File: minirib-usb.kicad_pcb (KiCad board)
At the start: 2 copper layers, 79.5 x 23 mm, 59 parts, among them J1 USB_B_Micro, J2 Mini-DIN-6-Shielded, J3 RS232, Q1 MMBT3906, Q2 MMBT3904, Q3 MMBT3904, Q4 MMBT3904, Q5 MMBT3906, Q6 MMBT3904, Q7 MMBT3904, Q8 BSS138W, U1 FT231XS, U2 TL071, U3 MAX232

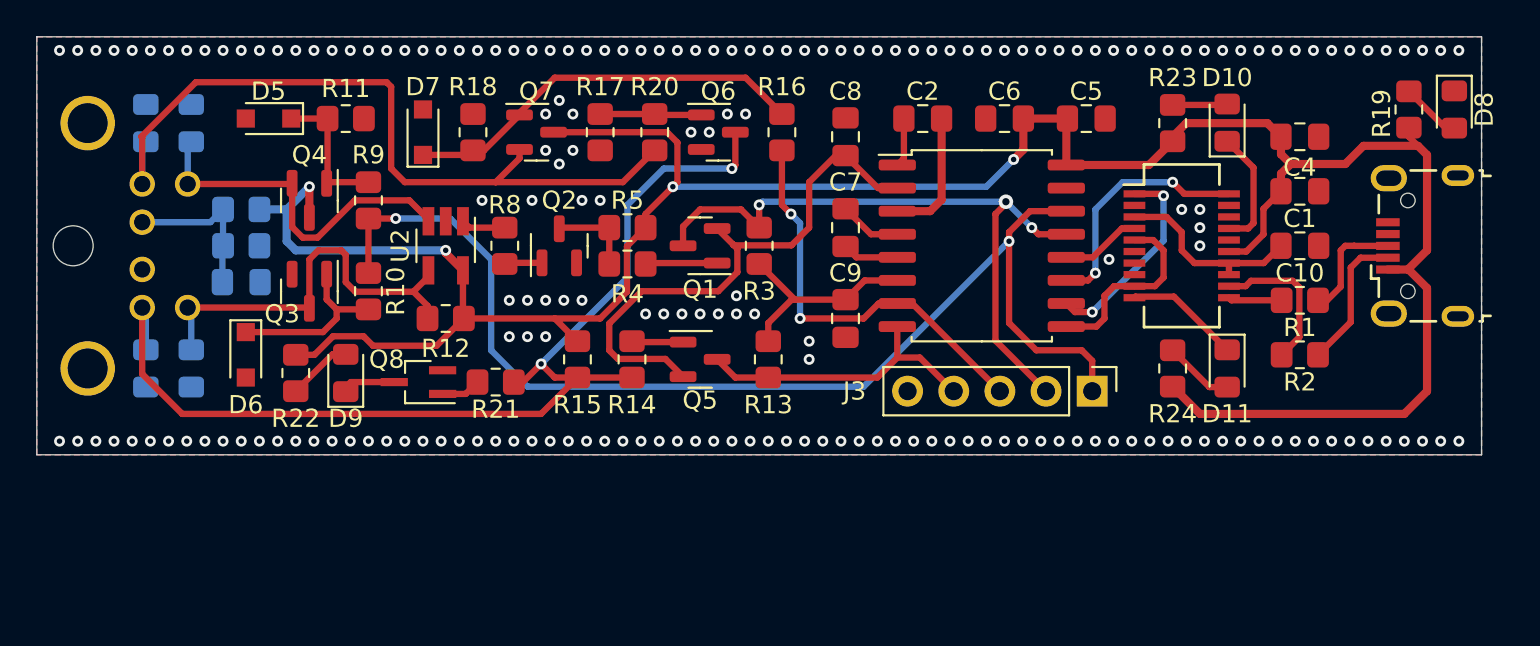
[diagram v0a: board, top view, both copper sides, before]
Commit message: initial revision D updates
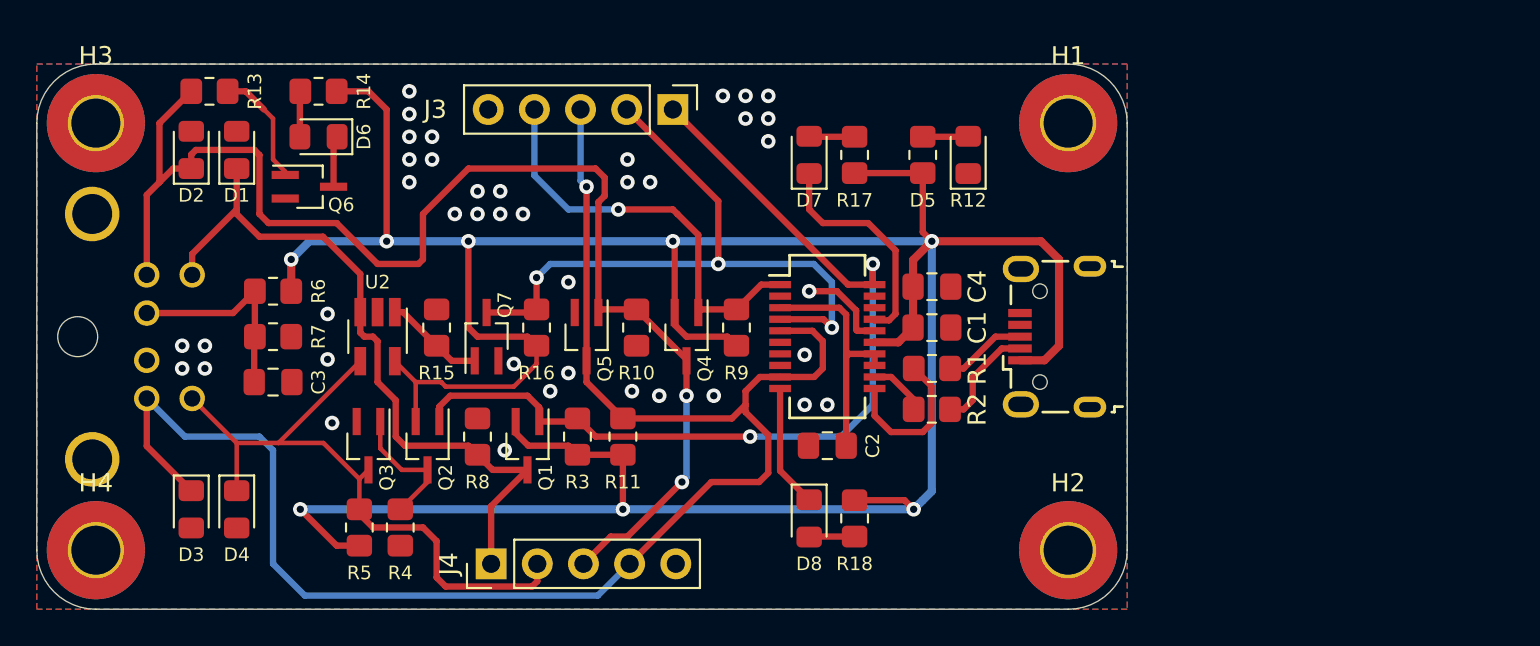
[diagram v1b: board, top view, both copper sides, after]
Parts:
- removed C10, C5: 0.1uF, Capacitor_SMD:C_0805_2012Metric_Pad1.18x1.45mm_HandSolder
- removed C6, C7, C8, C9: 1uF, Capacitor_SMD:C_0805_2012Metric_Pad1.18x1.45mm_HandSolder
- removed D10: TXD, Diode_SMD:D_0805_2012Metric_Pad1.15x1.40mm_HandSolder
- removed D11: RXD, Diode_SMD:D_0805_2012Metric_Pad1.15x1.40mm_HandSolder
- removed D9: BUSY, Diode_SMD:D_0805_2012Metric_Pad1.15x1.40mm_HandSolder
- removed Q8: BSS138W, Package_TO_SOT_SMD:SOT-323_SC-70_Handsoldering
- removed R19, R21, R22, R23, R24: 1k5, Resistor_SMD:R_0805_2012Metric_Pad1.20x1.40mm_HandSolder
- removed R20: 10k, Resistor_SMD:R_0805_2012Metric_Pad1.20x1.40mm_HandSolder
- removed U3: MAX232, Package_SO:SOIC-16W_7.5x10.3mm_P1.27mm
- added G***: LOGO, w3axl-logos:logo-6.3x6.3, B.Cu at (110.2, 115.8)
- added H1: MountingHole_Pad, MountingHole:MountingHole_2.7mm_M2.5_Pad_TopBottom, F.Cu at (156.8, 93.2)
- added H2: MountingHole_Pad, MountingHole:MountingHole_2.7mm_M2.5_Pad_TopBottom, F.Cu at (156.8, 116.8)
- added H3: MountingHole_Pad, MountingHole:MountingHole_2.7mm_M2.5_Pad_TopBottom, F.Cu at (103.2, 93.2)
- added H4: MountingHole_Pad, MountingHole:MountingHole_2.7mm_M2.5_Pad_TopBottom, F.Cu at (103.2, 116.8)
- added J4: UART, Connector_PinHeader_2.54mm:PinHeader_1x05_P2.54mm_Vertical, F.Cu at (125.0, 117.5)
- C2: value 1uF -> 0.1uF
- C3, D1, D2, D3, D4, R6, R7: moved to F.Cu
- D5: value 1N4148 -> PWR; footprint Diode_SMD:D_SOD-323_HandSoldering -> Diode_SMD:D_0805_2012Metric_Pad1.15x1.40mm_HandSolder
- D6: value 1N4148 -> BUSY; footprint Diode_SMD:D_SOD-323_HandSoldering -> Diode_SMD:D_0805_2012Metric_Pad1.15x1.40mm_HandSolder
- D7: value 1N4148 -> TXD; footprint Diode_SMD:D_SOD-323_HandSoldering -> Diode_SMD:D_0805_2012Metric_Pad1.15x1.40mm_HandSolder
- D8: value PWR -> RXD
- J3: value RS232 -> UART
- Q1: value MMBT3906 -> BS84W; footprint Package_TO_SOT_SMD:SOT-23 -> Package_TO_SOT_SMD:SOT-323_SC-70_Handsoldering
- Q2, Q4: value MMBT3904 -> BS84W; footprint Package_TO_SOT_SMD:SOT-23 -> Package_TO_SOT_SMD:SOT-323_SC-70_Handsoldering
- Q3, Q6, Q7: value MMBT3904 -> BSS138W; footprint Package_TO_SOT_SMD:SOT-23 -> Package_TO_SOT_SMD:SOT-323_SC-70_Handsoldering
- Q5: value MMBT3906 -> BSS138W; footprint Package_TO_SOT_SMD:SOT-23 -> Package_TO_SOT_SMD:SOT-323_SC-70_Handsoldering
- R10, R9: value 9k1 -> 10k
- R11: value 47k -> 10k
- R12, R14: value 10k -> 1k5
- R13, R3: value 1k5 -> 10k
- R16: value 4k7 -> 10k
- R17: value 4k7 -> 1k5
- R18: value 20k -> 1k5
- R8: value 20k -> 10k
- moved D8 42.0 mm to (142.5, 115.0)
- moved D5 38.6 mm to (151.2, 95.0), turned to 90 degrees
- moved R13 34.1 mm to (109.5, 91.5), turned to 0 degrees
- moved R18 29.9 mm to (145.0, 115.0)
- moved J3 27.8 mm to (135.0, 92.5)
- moved R12 27.8 mm to (148.8, 95.0), turned to -90 degrees
- moved R11 23.2 mm to (132.2, 110.5), turned to 90 degrees
- moved Q6 22.7 mm to (115.0, 96.8)
- moved R14 22.7 mm to (115.5, 91.5), turned to 0 degrees
- moved R5 22.1 mm to (117.8, 115.5), turned to 90 degrees
- moved Q4 22.1 mm to (135.8, 105.0)
- moved C4 21.9 mm to (149.3, 102.2)
- moved C1 21.6 mm to (149.3, 104.5)
- moved R9 21.4 mm to (138.5, 104.5)
- moved D7 21.3 mm to (142.5, 95.0)
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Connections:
- C2 pad 2: Net-(C2-Pad2) -> GND
- D5 pad 1: Net-(D5-Pad1) -> GND
- D5 pad 2: GND -> Net-(D5-Pad2)
- D6 pad 2: GND -> Net-(D6-Pad2)
- D7 pad 1: Net-(D7-Pad1) -> ~{TXLED}
- D7 pad 2: GND -> Net-(D7-Pad2)
- D8 pad 1: GND -> ~{RXLED}
- J3 pad 3: DTR -> BUSY
- J3 pad 4: CTS -> ~{DTR}
- Q1 pad 1: Net-(Q1-Pad1) -> TXD
- Q1 pad 2: +8V -> +5V
- Q1 pad 3: RXD -> BUS-
- Q2 pad 1: Net-(Q2-Pad1) -> TXD
- Q2 pad 2: GND -> +5V
- Q3 pad 1: Net-(D6-Pad1) -> Net-(Q2-Pad3)
- Q4 pad 1: Net-(D5-Pad1) -> ~{DTR}
- Q4 pad 2: BUS- -> +5V
- Q4 pad 3: +5V -> ~{BUSY}
- Q5 pad 1: Net-(Q5-Pad1) -> ~{BUSY}
- Q5 pad 2: +8V -> GND
- Q5 pad 3: CTS -> BUSY
- Q6 pad 3: BUSY -> Net-(D6-Pad1)
- Q7 pad 1: Net-(D7-Pad1) -> Net-(Q7-Pad1)
- Q7 pad 2: ~{BUSY} -> GND
- Q7 pad 3: +5V -> RXD
- R10 pad 1: Net-(D6-Pad1) -> GND
- R10 pad 2: TXD -> ~{BUSY}
- R11 pad 1: Net-(D5-Pad1) -> +5V
- R11 pad 2: GND -> BUSY
- R12 pad 1: +5V -> Net-(D5-Pad2)
- R12 pad 2: BUS+ -> +5V
- R13 pad 1: CTS -> ~{BUSY}
- R13 pad 2: -8V -> Net-(Q6-Pad1)
- R14 pad 1: BUSY -> Net-(D6-Pad2)
- R14 pad 2: Net-(Q5-Pad1) -> +5V
- R15 pad 1: BUSY -> Net-(Q7-Pad1)
- R15 pad 2: +5V -> GND
- R16 pad 1: Net-(D7-Pad1) -> RXD
- R16 pad 2: DTR -> +5V
- R17 pad 1: Net-(Q6-Pad1) -> Net-(D7-Pad2)
- R17 pad 2: GND -> +5V
- R18 pad 1: Net-(D7-Pad1) -> Net-(D8-Pad2)
- R18 pad 2: GND -> +5V
- R3 pad 1: RXD -> TXD
- R3 pad 2: -8V -> +5V
- R4 pad 1: Net-(Q1-Pad1) -> GND
- R5 pad 2: Net-(Q2-Pad3) -> BUS+
- R8 pad 1: Net-(R8-Pad1) -> GND
- R8 pad 2: Net-(Q2-Pad1) -> BUS-
- R9 pad 1: Net-(D5-Pad1) -> ~{DTR}
- R9 pad 2: TXD -> +5V
- U1 pad 1: ~{DTR_TTL} -> ~{DTR}
- U1 pad 13: Net-(C10-Pad1) -> Net-(C2-Pad1)
- U1 pad 14: Net-(C10-Pad1) -> Net-(C2-Pad1)
- U1 pad 20: TXD_TTL -> TXD
- U1 pad 3: Net-(C10-Pad1) -> Net-(C2-Pad1)
- U1 pad 4: RXD_TTL -> RXD
- U1 pad 5: ~{CTS_TTL} -> BUSY
- U1 pad 9: ~{CTS_TTL} -> BUSY
- U2 pad 1: Net-(R8-Pad1) -> Net-(Q7-Pad1)
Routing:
- net BUSY: track 58.3 -> 90.1 mm, vias 2 -> 1
- net +8V: track 30.5 -> 0.00 mm
- net ~{BUSY}: track 42.5 -> 72.9 mm, vias 0 -> 2
- net +5V: track 146.1 -> 173.8 mm, vias 4 -> 8
- net ~{DTR}: track 0.00 -> 23.4 mm, vias 0 -> 1
- net DTR: track 23.0 -> 0.00 mm, vias 2 -> 0
- net Net-(D7-Pad1): track 22.4 -> 0.00 mm
- net BUS-: track 19.7 -> 39.3 mm
- net CTS: track 16.7 -> 0.00 mm
- net TXD_TTL: track 13.5 -> 0.00 mm, vias 2 -> 0
- net BUS+: track 22.9 -> 36.3 mm
- net TXD: track 64.1 -> 51.2 mm
- net -8V: track 11.8 -> 0.00 mm
- net ~{DTR_TTL}: track 11.3 -> 0.00 mm, vias 2 -> 0
- net Net-(C10-Pad1): track 10.7 -> 0.00 mm
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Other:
- board size 79.5 x 23 mm -> 60 x 30 mm
- board text added: "MiniRIB USB Rev D"
